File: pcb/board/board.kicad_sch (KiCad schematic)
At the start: 121 parts, among them J1 (A) USB_C_Receptacle_USB2.0_1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, J10 OLED_128x32, J11 LCD_128x160, J12 AudioJack2, J13 AudioJack3, J14 Micro_SD_Card, J2 (B) USB_C_Receptacle_USB2.0_1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, J3 (C) USB_C_Receptacle_USB2.0_1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, J4 Conn_01x03, J5 Conn_01x03, J6 Conn_01x20, J7 Conn_01x20, J8 Conn_01x20, J9 Conn_01x20, SW1 SW_Push, SW2 SW_Push, SW3 Switch, SW4 Switch, SW5 Switch, SW6 RotaryEncoder_Switch, U1 RP2040, U2 NCP1117-3.3_SOT223, U3 W25Q128JVS, U4 NCP1117-3.3_SOT223, U5 RP2040, U6 W25Q128JVS, U7 PCM5101A, U8 TLV70033_SOT23-5, U9 TPA6132A2RTE, Y1 12MHz, Y2 12MHz

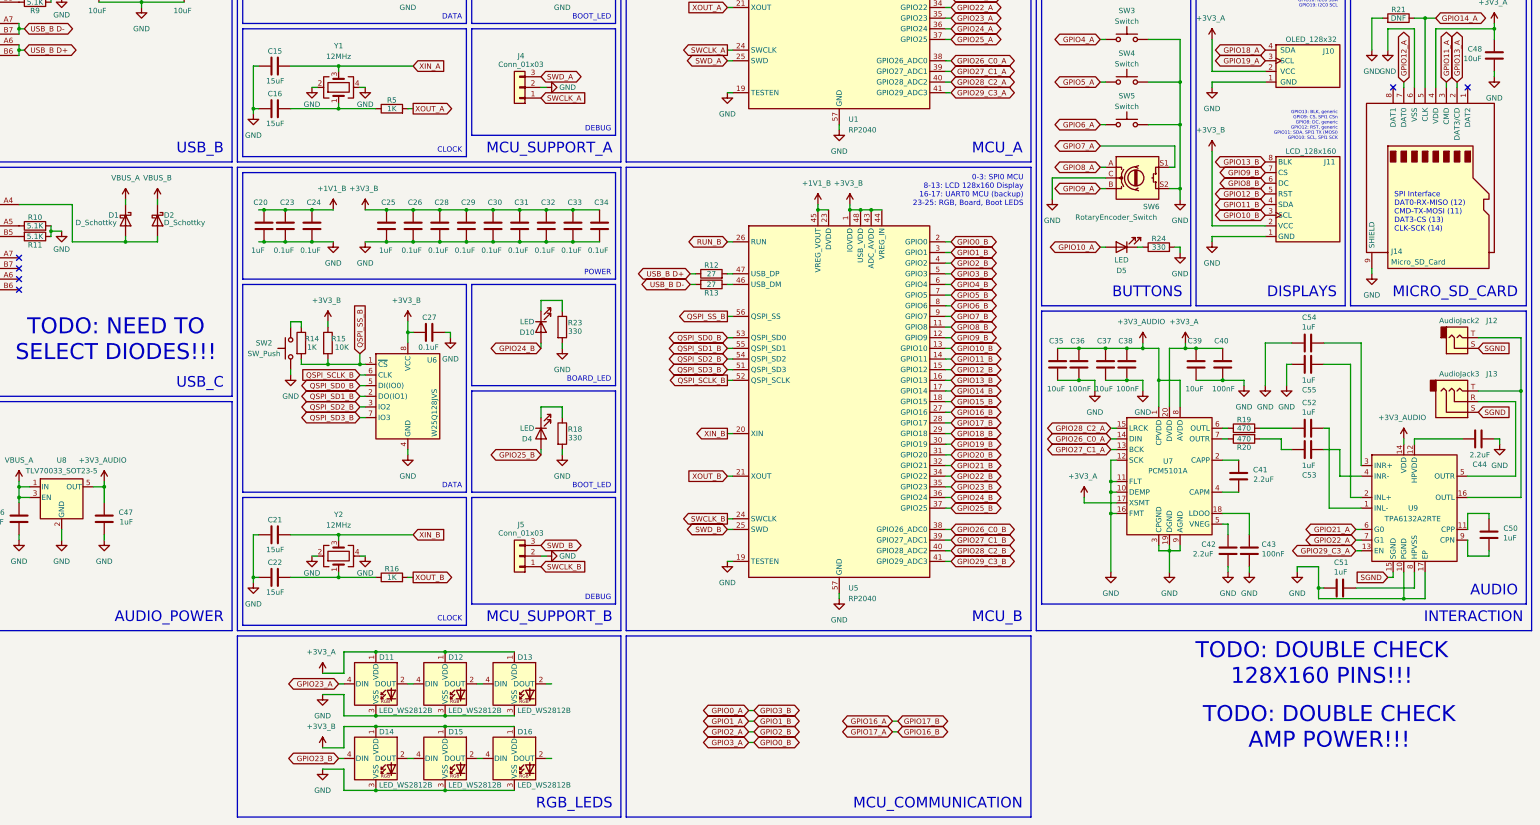
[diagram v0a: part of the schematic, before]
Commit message: footprint assigning and wrapping up schematic work!
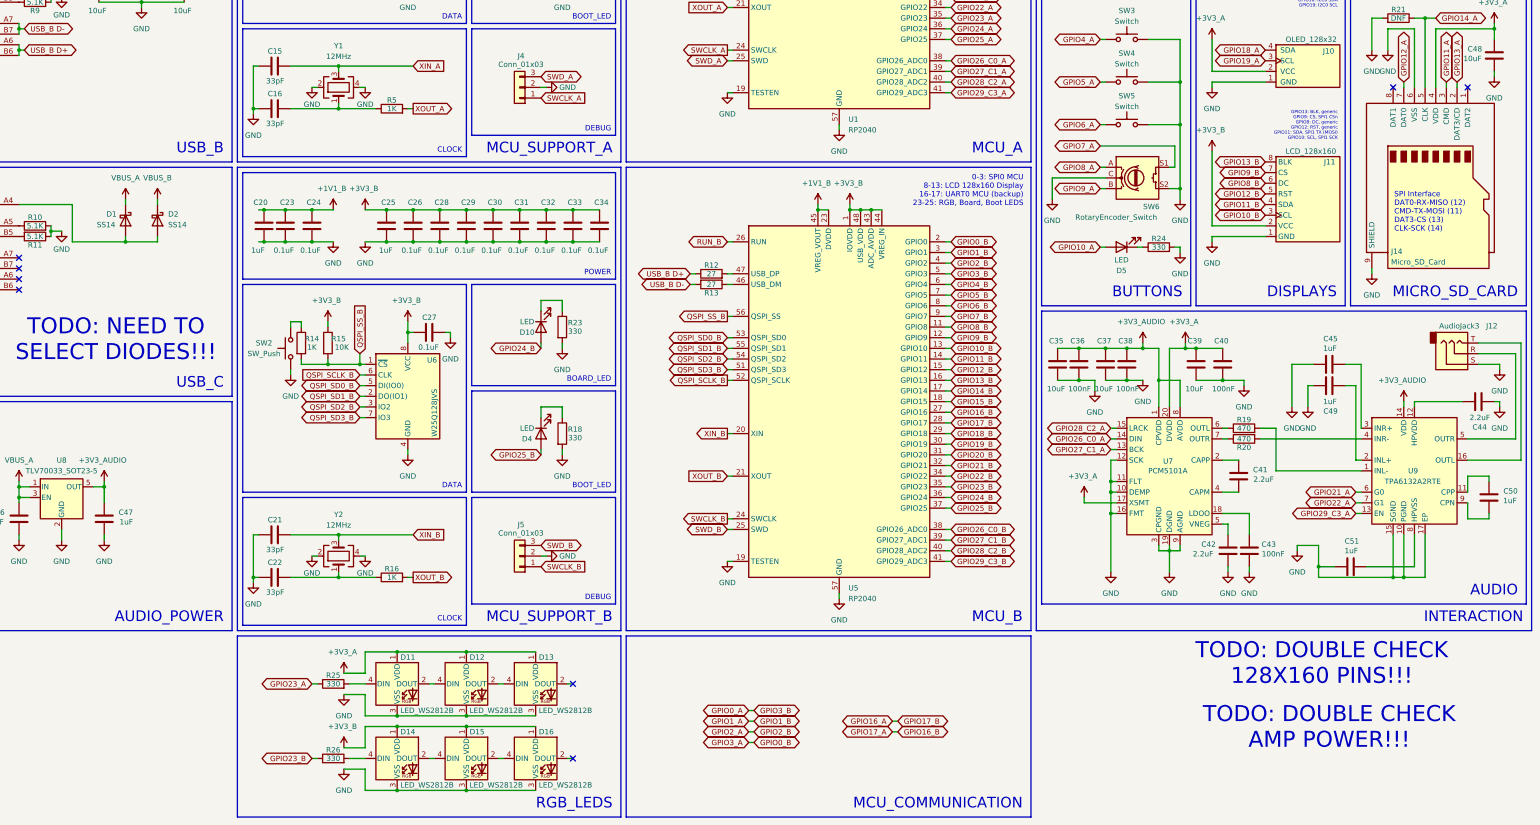
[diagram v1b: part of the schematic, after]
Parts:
- removed C52, C53, C54, C55: 1uF, Capacitor_SMD:C_0402_1005Metric, symbol Device:C
- removed D1, D2: D_Schottky, symbol Device:D_Schottky
- removed J12: AudioJack2, symbol Connector_Audio:AudioJack2
- added C45, C49: 1uF, Capacitor_SMD:C_0603_1608Metric, symbol Device:C
- added D1, D2: SS14, Diode_SMD:D_SMA, symbol Diode:SS14
- added R25, R26: 330, Resistor_SMD:R_0402_1005Metric, symbol Device:R
- C1, C10, C11, C12, C13, C14, C17, C18, C19, C2, C20, C23, C24, C25, C26, C27, C28, C29, C3, C30, C31, C32, C33, C34, C35, C36, C37, C38, C39, C4, C40, C41, C42, C43, C44, C46, C47, C48, C5, C50, C51, C6, C7, C8, C9: footprint Capacitor_SMD:C_0402_1005Metric -> Capacitor_SMD:C_0603_1608Metric
- C15, C16, C21, C22: value 15uF -> 33pF; footprint Capacitor_SMD:C_0402_1005Metric -> Capacitor_SMD:C_0603_1608Metric
- D10, D3, D4, D5, D9: footprint (none) -> LED_SMD:LED_0603_1608Metric
- J12: renamed from J13; footprint (none) -> Connector_Audio:Jack_3.5mm_CUI_SJ-3523-SMT_Horizontal
- J14: footprint (none) -> Connector_Card:microSD_HC_Wuerth_693072010801
- SW6: footprint Rotary_Encoder:RotaryEncoder_Alps_EC11E_Vertical_H20mm -> Rotary_Encoder:RotaryEncoder_Alps_EC11E-Switch_Vertical_H20mm
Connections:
- net SGND is gone; now on net GND: J12.S, U9.15 (SGND)
- net GND: now also C45.1, C49.1
- net GPIO23_A: now also R25.1; no longer D11.4 (DIN)
- net GPIO23_B: now also R26.1; no longer D14.4 (DIN)
- net VBUS_A: now also D1.1 (K)
- net VBUS_B: now also D2.1 (K)
- net at R19.2: now also U9.1 (INL-)
- net at R20.2: now also U9.4 (INR-)
- net at U9.2 (INL+): now also C49.2
- net at J3.A4 (VBUS), J3.A9 (VBUS), J3.B4 (VBUS)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: now also D1.2 (A), D2.2 (A)
- net at U9.3 (INR+): now also C45.2
- new net: D11.4 (DIN), R25.2
- new net: D14.4 (DIN), R26.2
- no-connect marks 6 -> 8
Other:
- moved on the sheet: C44, C50, C51, D11, D12, D13, D14, D15, D16, J12, U9
